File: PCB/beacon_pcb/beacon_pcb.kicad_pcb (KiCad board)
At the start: 2 copper layers, 19 x 18 mm, 6 parts, among them P1 CONN_01X02

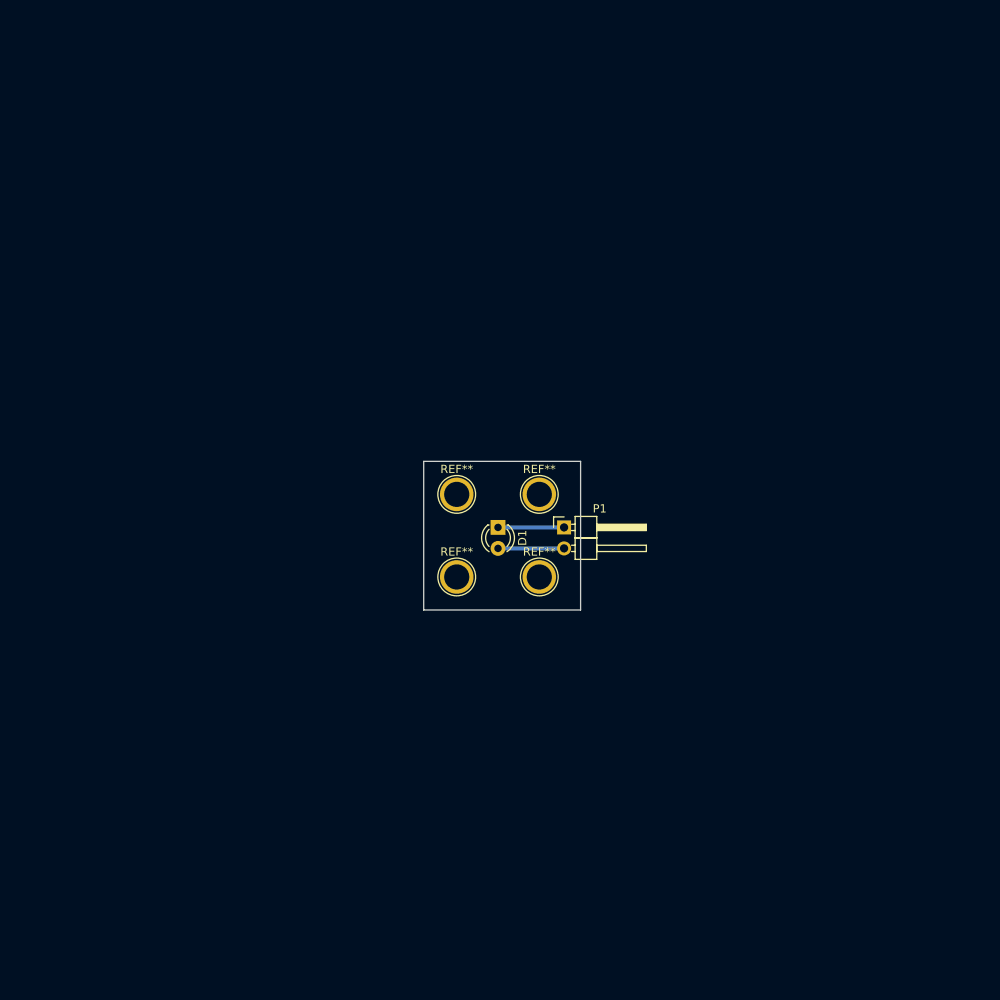
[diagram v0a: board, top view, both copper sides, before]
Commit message: Debugging tweaks
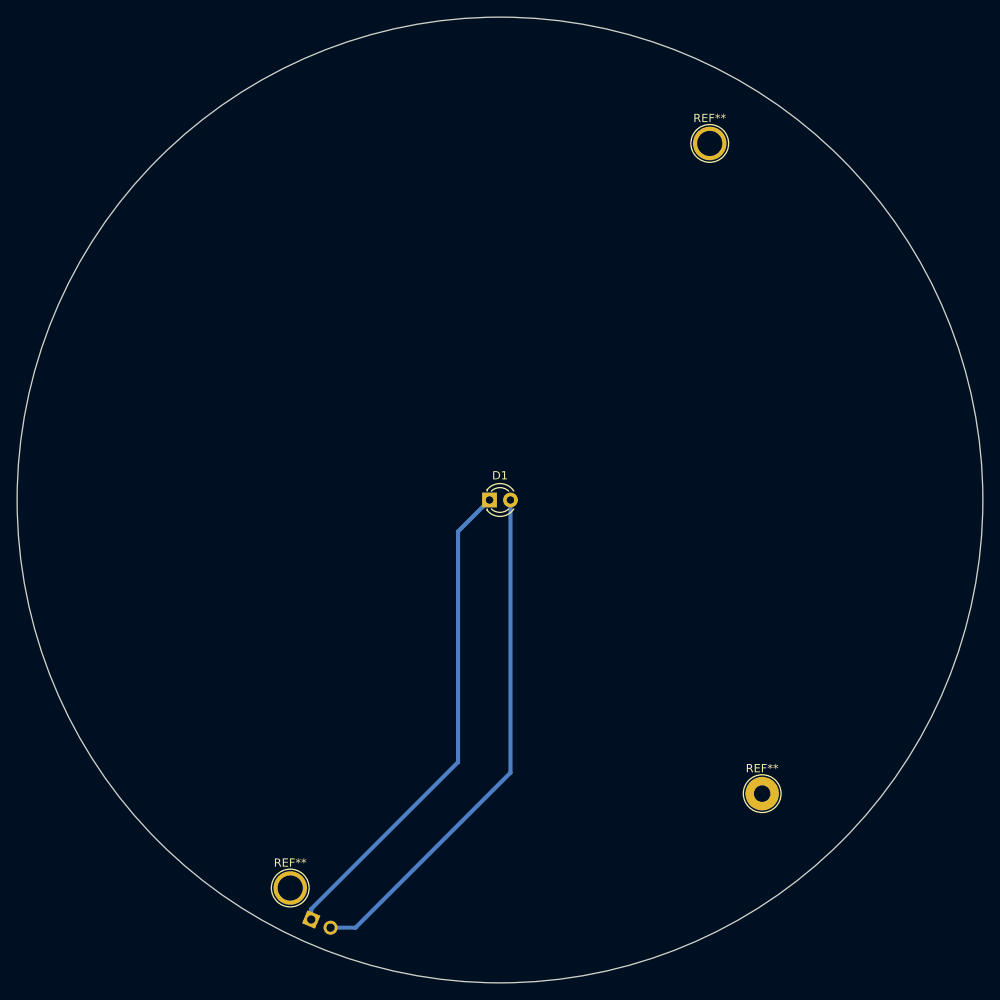
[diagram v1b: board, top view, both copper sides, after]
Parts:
- removed the REF** at (137.0, 116.0)
- removed the REF** at (137.0, 106.0)
- added REF**: 1pin, Connect:1pin, F.Cu at (174.0, 142.2)
- P1: moved to B.Cu
- moved P1 56.5 mm to (119.4, 157.5), turned to 247 degrees
- moved REF** 48.3 mm to (116.8, 153.7)
- moved REF** 47.2 mm to (167.6, 63.5)
- moved D1 3.48 mm to (141.0, 106.7), turned to 0 degrees
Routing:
- net Net-(D1-Pad2): track 8.00 -> 62.6 mm
- net Net-(D1-Pad1): track 8.00 -> 59.7 mm
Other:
- board size 19 x 18 mm -> 117 x 117 mm
